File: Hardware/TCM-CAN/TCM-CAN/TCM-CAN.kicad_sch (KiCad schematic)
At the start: 6 parts, among them J2 Conn_01x27_Socket, J3 Conn_01x27_Socket, J4 Conn_02x20_Odd_Even, J5 Conn_01x06_Socket

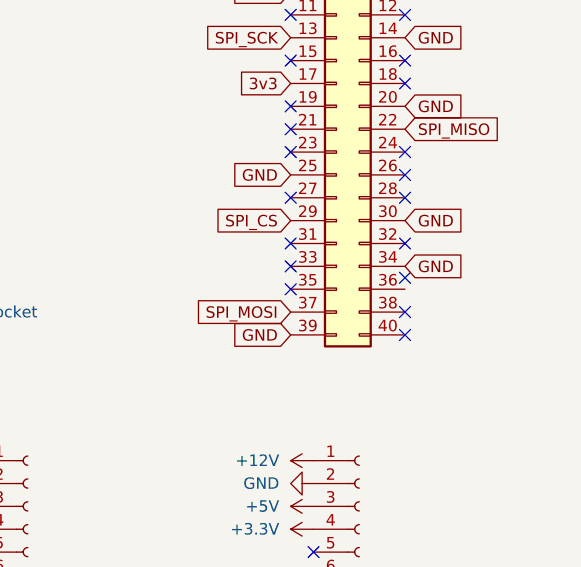
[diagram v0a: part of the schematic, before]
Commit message: tcm-can pcb done
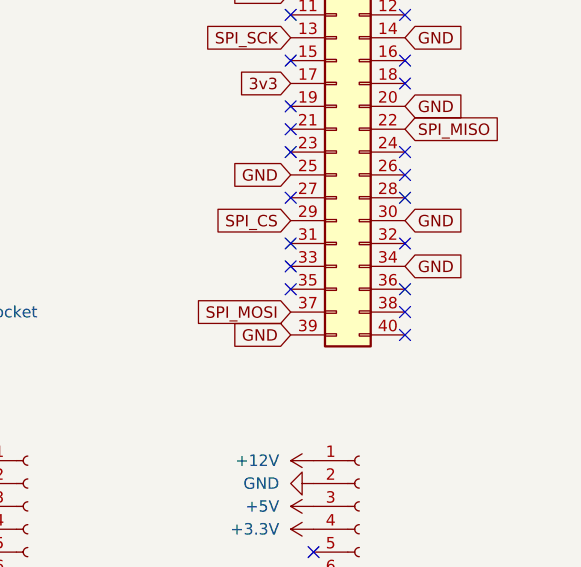
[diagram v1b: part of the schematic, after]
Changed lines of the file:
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@@
 	)
 	(no_connect
-		(at 227.33 62.23)
+		(at 227.33 63.5)
 	)
 	(no_connect
@@
 			"Ki5DdSIgIiouTWFzayIpKHJlbW92ZV91bnVzZWRfbGF5ZXJzIG5vKShuZXQgNTQgIlNQSV9NSVNP"
 			"IikocGluZnVuY3Rpb24gIlBpbl8yMiIpKHBpbnR5cGUgInBhc3NpdmUiKSh1dWlkICI5NzVlOGVl"
-			"Yi0zY2U3LTQ4M2ItYjhkNi0zZjkwODg2NGM1Zg=="
+			"Yi0zY2U3LTQ4M2ItYjhkNi0zZjkwODg2NGM1Zv//CCQAAHcSAAASAAAAdxIAABIAAAD/////ACQA"
+			"AIkSAAAYAAAAiRIAABgAAAD/////ACQAAKESAAALAAAAoRIAAAsAAAD/////ACQAAKwSAAAUAAAA"
+			"rBIAABQAAAD/////CCQAAMASAAANAAAAwBIAAA0AAAD/////ACQAAM0SAAAIAAAAzRIAAAgAAAD/"
+			"////ACQAANUSAAAJAAAA1RIAAAkAAAD/////ACQAAN4SAAATAAAA3hIAABMAAAD/////CCQAAPES"
+			"AAAHAAAA8RIAAAcAAAD/////ACQAAPgSAAAIAAAA+BIAAAgAAAD/////ACQAAAATAAAIAAAAABMA"
+			"AAgAAAD/////ACQAAAgTAAATAAAACBMAABMAAAD/////CCQAABsTAAAIAAAAGxMAAAgAAAD/////"
+			"ACQAACMTAAAZAAAAIxMAABkAAAD/////ACQAADwTAAAPAAAAPBMAAA8AAAD/////ACQAAEsTAAAS"
+			"AAAASxMAABIAAAD/////ACQAAF0TAAASAAAAXRMAABIAAAD/////ACQAAG8TAAASAAAAbxMAABIA"
+			"AAD/////ACQAAIETAAAUAAAAgRMAABQAAAD/////ACQAAJUTAAATAAAAlRMAABMAAAD/////ACQA"
+			"AKgTAAAUAAAAqBMAABQAAAD/////ACQAALwTAAAIAAAAvBMAAAgAAAD/////ACQAAMQTAAAIAAAA"
+			"xBMAAAgAAAD/////ACQAAMwTAAAIAAAAzBMAAAgAAAD/////ACQAANQTAAAIAAAA1BMAAAgAAAD/"
+			"////ACQAANwTAAAIAAAA3BMAAAgAAAD/////ACQAAOQTAAAIAAAA5BMAAAgAAAD/////ACQAAOwT"
+			"AAAIAAAA7BMAAAgAAAD/////ACQAAPQTAAAIAAAA9BMAAAgAAAD/////ACQAAPwTAAAIAAAA/BMA"
+			"AAgAAAD/////ACQAAAQUAAAIAAAABBQAAAgAAAD/////ACQAAAwUAAAIAAAADBQAAAgAAAD/////"
+			"ACQAABQUAAAIAAAAFBQAAAgAAAD/////ACQAABwUAAAIAAAAHBQAAAgAAAD/////ACQAACQUAAAI"
+			"AAAAJBQAAAgAAAD/////ACQAACwUAAAIAAAALBQAAAgAAAD/////ACQAADQUAAAIAAAANBQAAAgA"
+			"AAD/////ACQAADwUAAAIAAAAPBQAAAgAAAD/////ACQAAEQUAAAIAAAARBQAAAgAAAD/////ACQA"
+			"AEwUAAAIAAAATBQAAAgAAAD/////ACQAAFQUAAAIAAAAVBQAAAgAAAD/////ACQAAFwUAAAIAAAA"
+			"XBQAAAgAAAD/////ACQAAGQUAAAIAAAAZBQAAA=="
 		)
 	)
